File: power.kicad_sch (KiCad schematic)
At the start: 35 parts, among them J4 USB_C_Receptacle_USB2.0_16P, J7 Ext VCC Out, U2 BQ25170DSGR, U5 TPS628438DRL

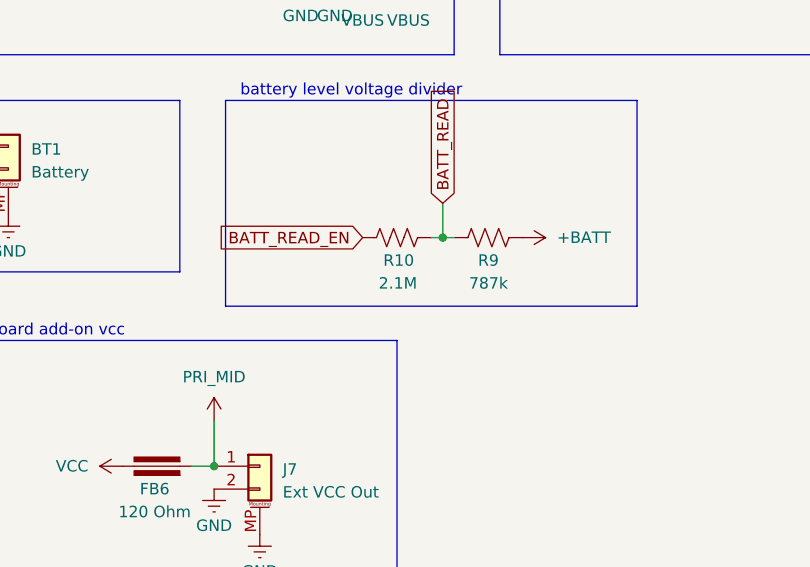
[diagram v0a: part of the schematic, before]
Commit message: actually production version, for real?
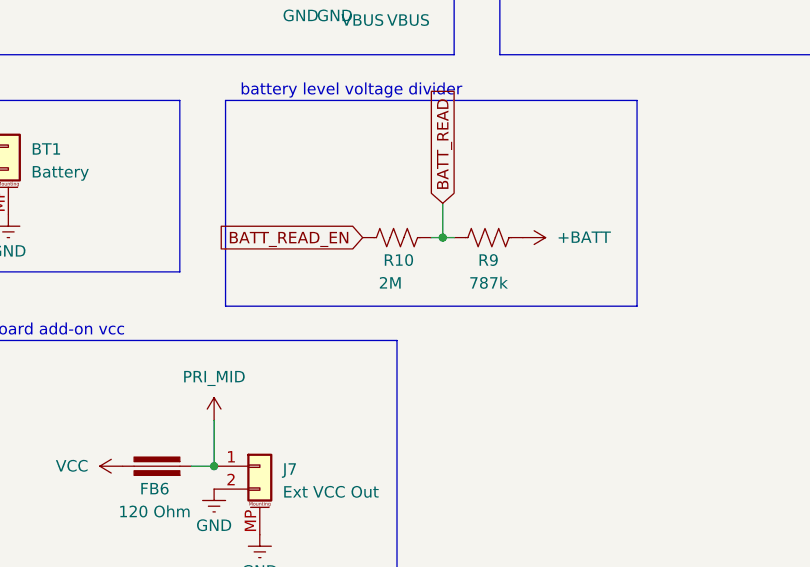
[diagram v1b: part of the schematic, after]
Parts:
- FB6: footprint PCM_Ferrite_SMD_AKL:Ferrite_0603_1608Metric -> PCM_Ferrite_SMD_AKL:Ferrite_0805_2012Metric
- R10: value 2.1M -> 2M
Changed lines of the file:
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@@
 			)
 		)
-		(property "Footprint" "PCM_Ferrite_SMD_AKL:Ferrite_0603_1608Metric"
+		(property "Footprint" "PCM_Ferrite_SMD_AKL:Ferrite_0805_2012Metric"
 			(at 137.16 116.332 0)
 			(effects
@@
 			)
 		)
-		(property "Value" "2.1M"
+		(property "Value" "2M"
 			(at 161.798 92.71 90)
 			(effects

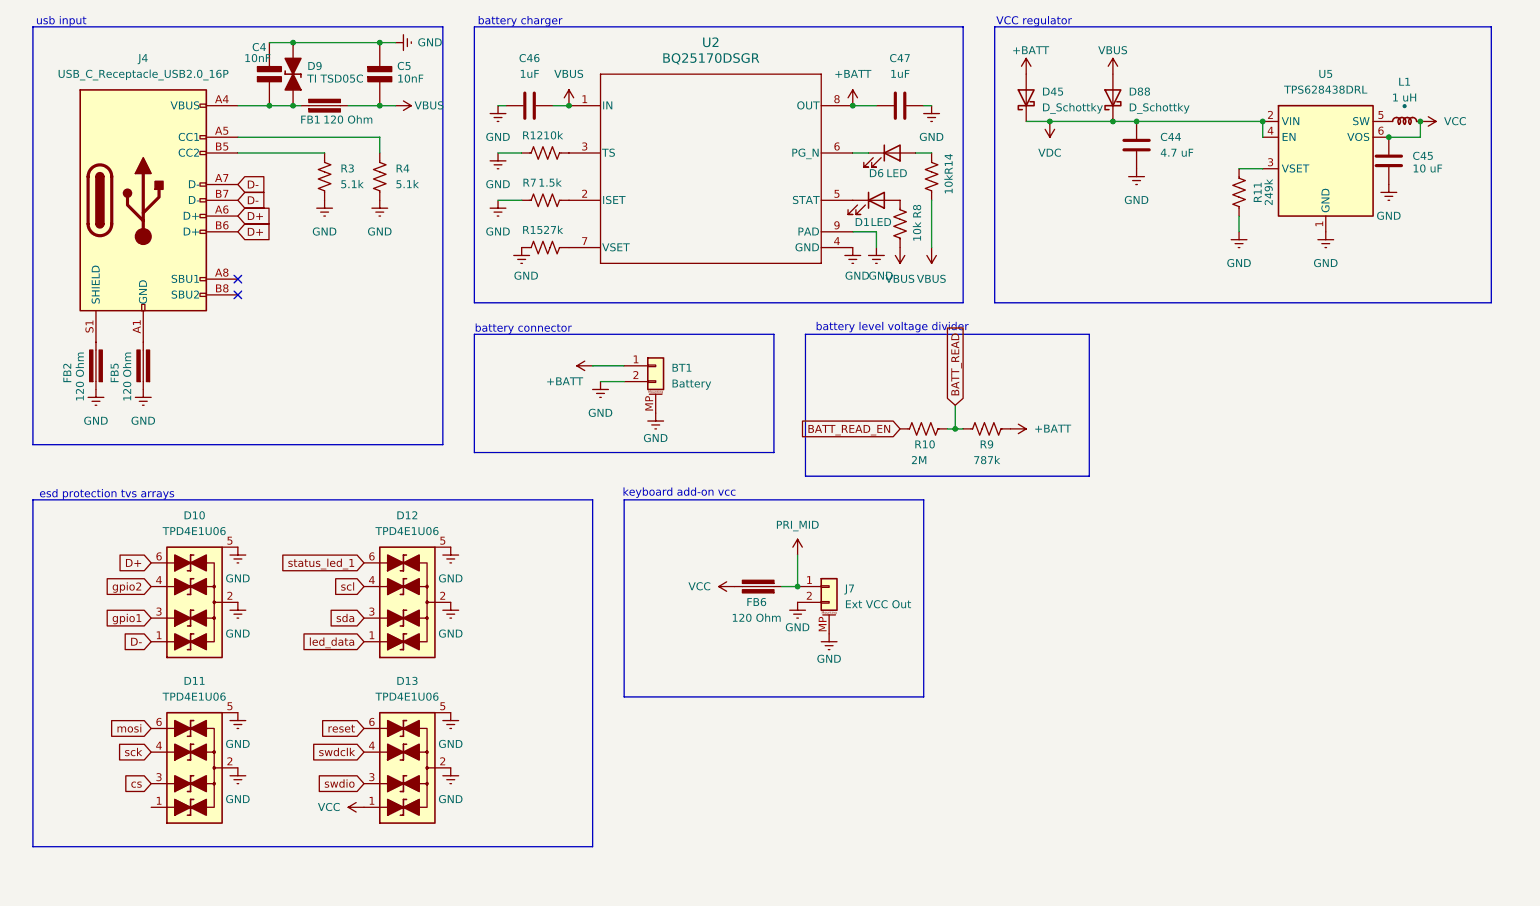
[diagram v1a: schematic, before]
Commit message: the final, actual, mk2 production files for real
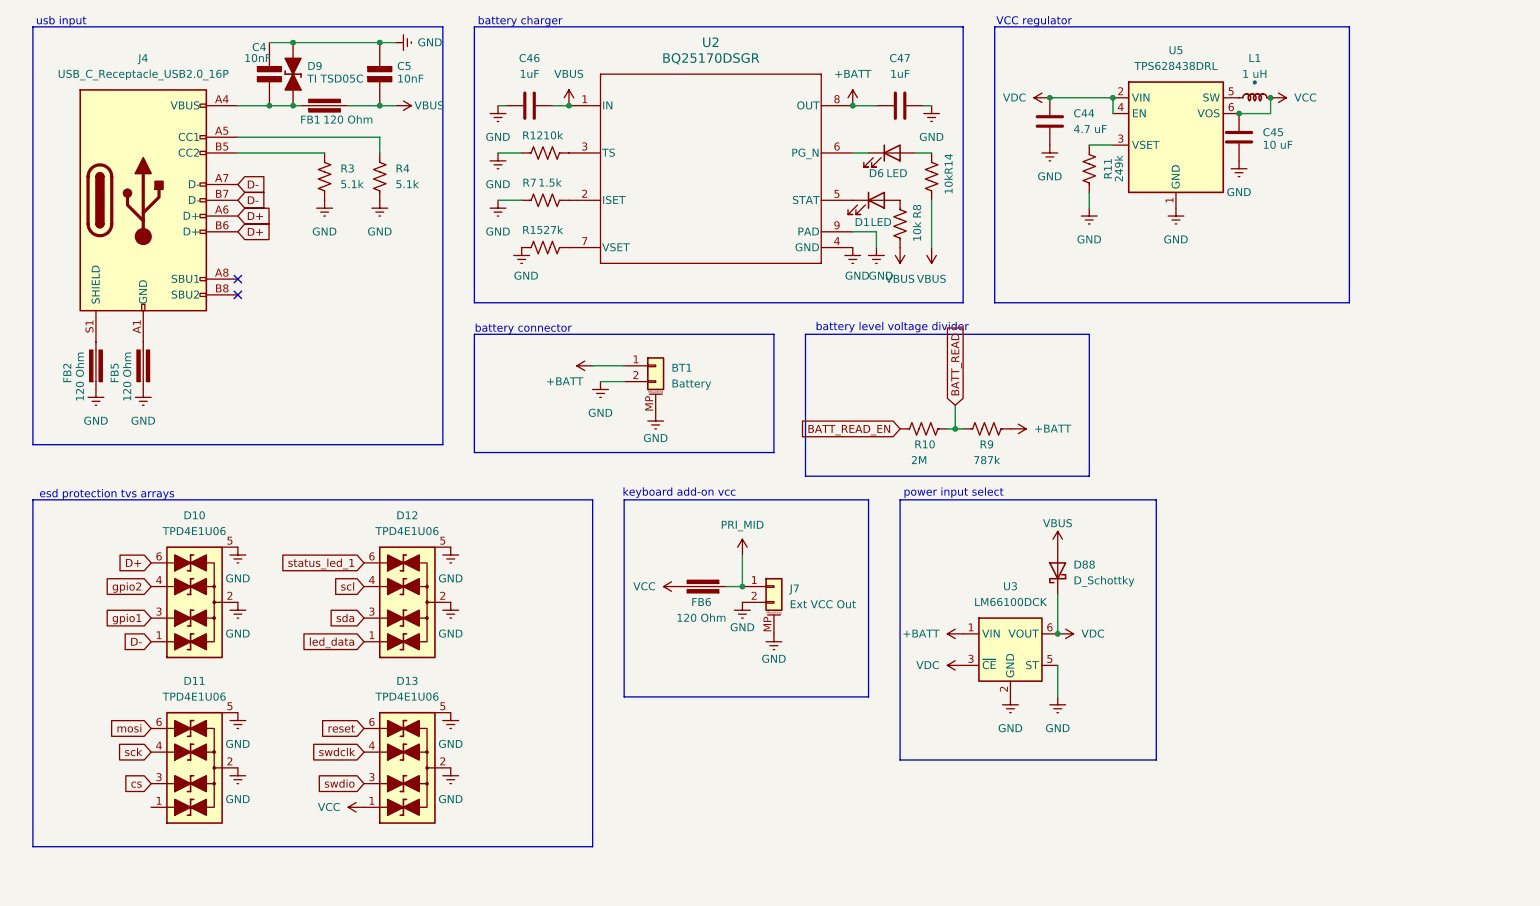
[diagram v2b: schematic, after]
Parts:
- removed D45: D_Schottky, PCM_Diode_SMD_Handsoldering_AKL:D_SOD-123F, symbol Device:D_Schottky
- added U3: LM66100DCK, Package_TO_SOT_SMD:SOT-363_SC-70-6, symbol Power_Management:LM66100DCK
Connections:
- net +BATT: now also U3.1 (VIN)
- net GND: now also U3.2 (GND), U3.5 (ST)
- net VDC: now also U3.3 (~{CE}), U3.6 (VOUT)
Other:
- note added: "power input select"
- moved on the sheet: C44, C45, D88, FB6, J7, L1, R11, U5

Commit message: mariposa v2 pre
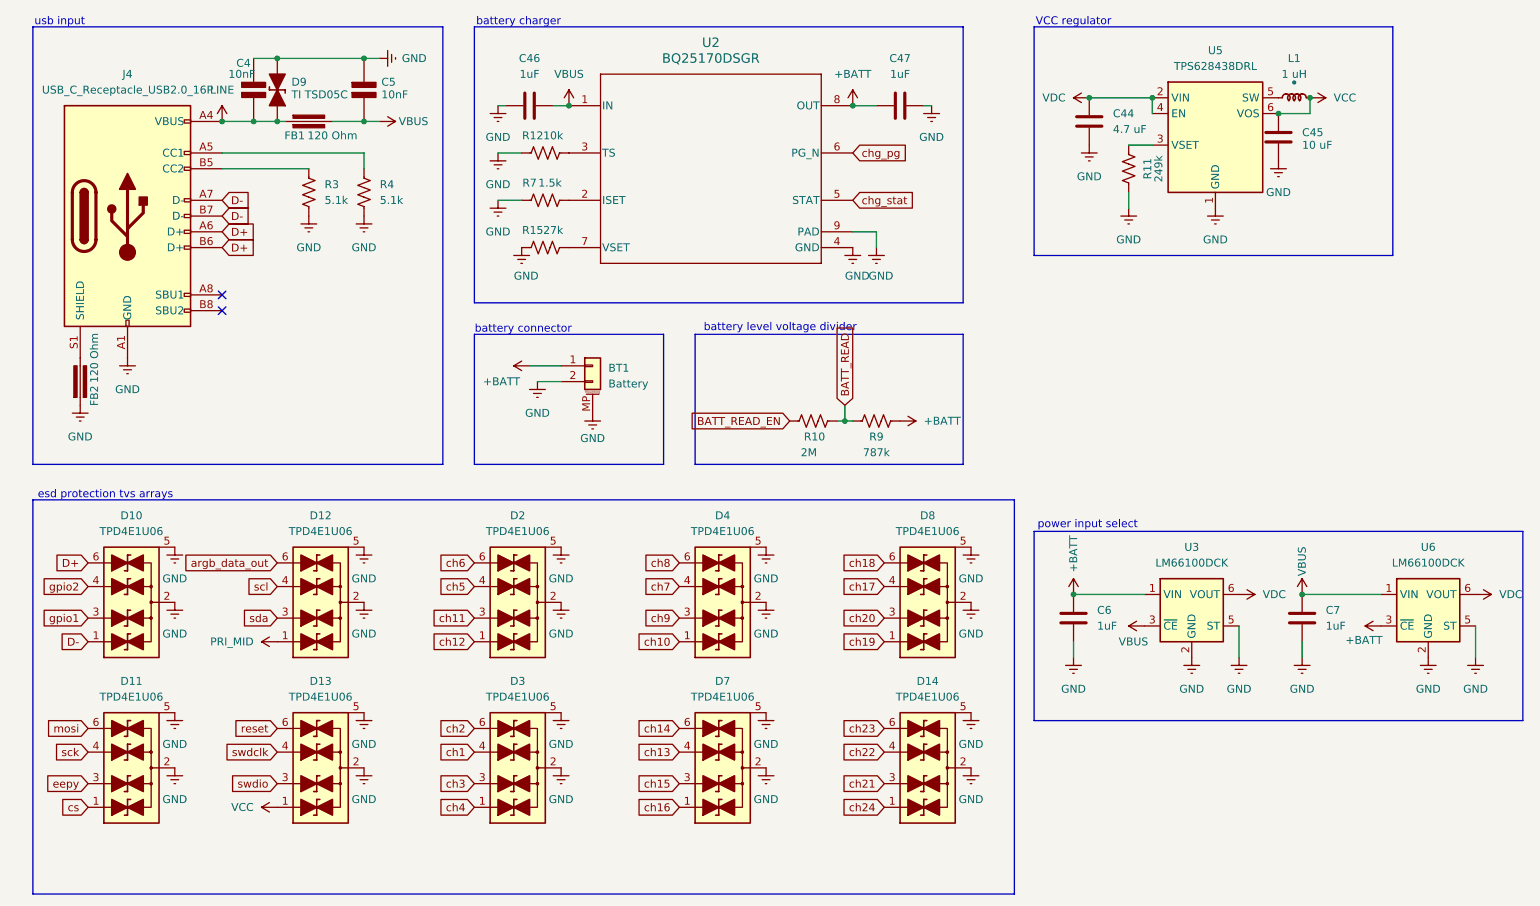
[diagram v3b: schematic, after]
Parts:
- removed D1, D6: LED, coquette_footprints:LED 1206 reverse mount rectangle, symbol Device:LED
- removed D88: D_Schottky, PCM_Diode_SMD_Handsoldering_AKL:D_SOD-123F, symbol Device:D_Schottky
- removed FB5, FB6: 120 Ohm, PCM_Ferrite_SMD_AKL:Ferrite_0805_2012Metric, symbol PCM_Device_AKL:Ferrite_Bead
- removed J7: Ext VCC Out, Connector_JST:JST_SUR_SM02B-SURS-TF_1x02-1MP_P0.80mm_Horizontal, symbol Connector_Generic_MountingPin:Conn_01x02_MountingPin
- removed R14, R8: 10k, Resistor_SMD:R_0603_1608Metric, symbol Device:R_US
- added C6, C7: 1uF, Capacitor_SMD:C_0603_1608Metric, symbol Device:C
- added D14, D2, D3, D4, D7, D8: TPD4E1U06, coquette_footprints:TPD4E1U06, symbol coquette_symbols:TPD4E1U06
- added U6: LM66100DCK, coquette_footprints:LM66100DCK, symbol Power_Management:LM66100DCK
- BT1: footprint Connector_JST:JST_GH_SM02B-GHS-TB_1x02-1MP_P1.25mm_Horizontal -> Connector_Molex:Molex_PicoBlade_53261-0271_1x02-1MP_P1.25mm_Horizontal
- C4, C5: footprint Capacitor_SMD:C_0603_1608Metric -> Capacitor_SMD:C_0402_1005Metric
- D10, D11, D12, D13: footprint PCM_Package_TO_SOT_SMD_AKL:SOT-363_SC-70-6 -> coquette_footprints:TPD4E1U06
- D9: footprint PCM_Diode_SMD_AKL:D_SOD-323_TVS -> coquette_footprints:TSD05C
- FB1, FB2: footprint PCM_Ferrite_SMD_AKL:Ferrite_0805_2012Metric -> PCM_Ferrite_SMD_AKL:Ferrite_1206_3216Metric
- U3: footprint Package_TO_SOT_SMD:SOT-363_SC-70-6 -> coquette_footprints:LM66100DCK
- U5: footprint Package_TO_SOT_SMD:SOT-563 -> coquette_footprints:TPS628438DRL
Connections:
- net led_data is gone; now on net PRI_MID: D12.1 (L1)
- net +BATT: now also C6.1, U6.3 (~{CE})
- net GND: now also J4.A1 (GND), J4.A12 (GND), J4.B1 (GND), J4.B12 (GND), C6.2, C7.2, D14.2 (VN), D14.5 (NC), D2.2 (VN), D2.5 (NC), D3.2 (VN), D3.5 (NC), D4.2 (VN), D4.5 (NC), D7.2 (VN), D7.5 (NC), D8.2 (VN), D8.5 (NC), U6.2 (GND), U6.5 (ST)
- net VBUS: now also U3.3 (~{CE}), C7.1, U6.1 (VIN)
- net VDC: now also U6.6 (VOUT); no longer U3.3 (~{CE})
- net cs: now also D11.1 (L1); no longer D11.3 (L2)
- net LINE: now reaches C4.2 (-), D9.2 (A), FB1.1, J4.A4 (VBUS), J4.A9 (VBUS), J4.B4 (VBUS), J4.B9 (VBUS)
- net chg_stat: now reaches U2.5 (STAT)
- net chg_pg: now reaches U2.6 (PG_N)
- net status_led_1 renamed argb_data_out
- new net ch1: D3.4 (L3)
- new net ch10: D4.1 (L1)
- new net ch11: D2.3 (L2)
- new net ch12: D2.1 (L1)
- new net ch13: D7.4 (L3)
- new net ch14: D7.6 (L4)
- new net ch15: D7.3 (L2)
- new net ch16: D7.1 (L1)
- new net ch17: D8.4 (L3)
- new net ch18: D8.6 (L4)
- new net ch19: D8.1 (L1)
- new net ch2: D3.6 (L4)
- new net ch20: D8.3 (L2)
- new net ch21: D14.3 (L2)
- new net ch22: D14.4 (L3)
- new net ch23: D14.6 (L4)
- new net ch24: D14.1 (L1)
- new net ch3: D3.3 (L2)
- new net ch4: D3.1 (L1)
- new net ch5: D2.4 (L3)
- new net ch6: D2.6 (L4)
- new net ch7: D4.4 (L3)
- new net ch8: D4.6 (L4)
- new net ch9: D4.3 (L2)
- new net eepy: D11.3 (L2)
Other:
- note removed: "keyboard add-on vcc"
- moved on the sheet: BT1, C4, C44, C45, C5, D10, D11, D12, D13, D9, FB1, J4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
